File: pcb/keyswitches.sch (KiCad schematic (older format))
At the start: 59 parts, among them J5 Conn_01x05, J6 Conn_01x03, SW1 SW_PUSH, SW10 SW_PUSH, SW11 SW_PUSH, SW12 SW_PUSH, SW13 SW_PUSH, SW14 SW_PUSH, SW15 SW_PUSH, SW16 SW_PUSH, SW17 SW_PUSH, SW18 SW_PUSH, SW19 SW_PUSH, SW2 SW_PUSH, SW20 SW_PUSH, SW21 SW_PUSH, SW22 SW_PUSH, SW23 SW_PUSH, SW24 SW_PUSH, SW25 SW_PUSH, SW26 SW_PUSH, SW27 SW_PUSH, SW28 Rotary_Encoder, SW29 Rotary_Encoder, SW3 SW_PUSH, SW30 Rotary_Encoder, SW4 SW_PUSH, SW5 SW_PUSH, SW6 SW_PUSH, SW7 SW_PUSH, SW8 SW_PUSH, SW9 SW_PUSH

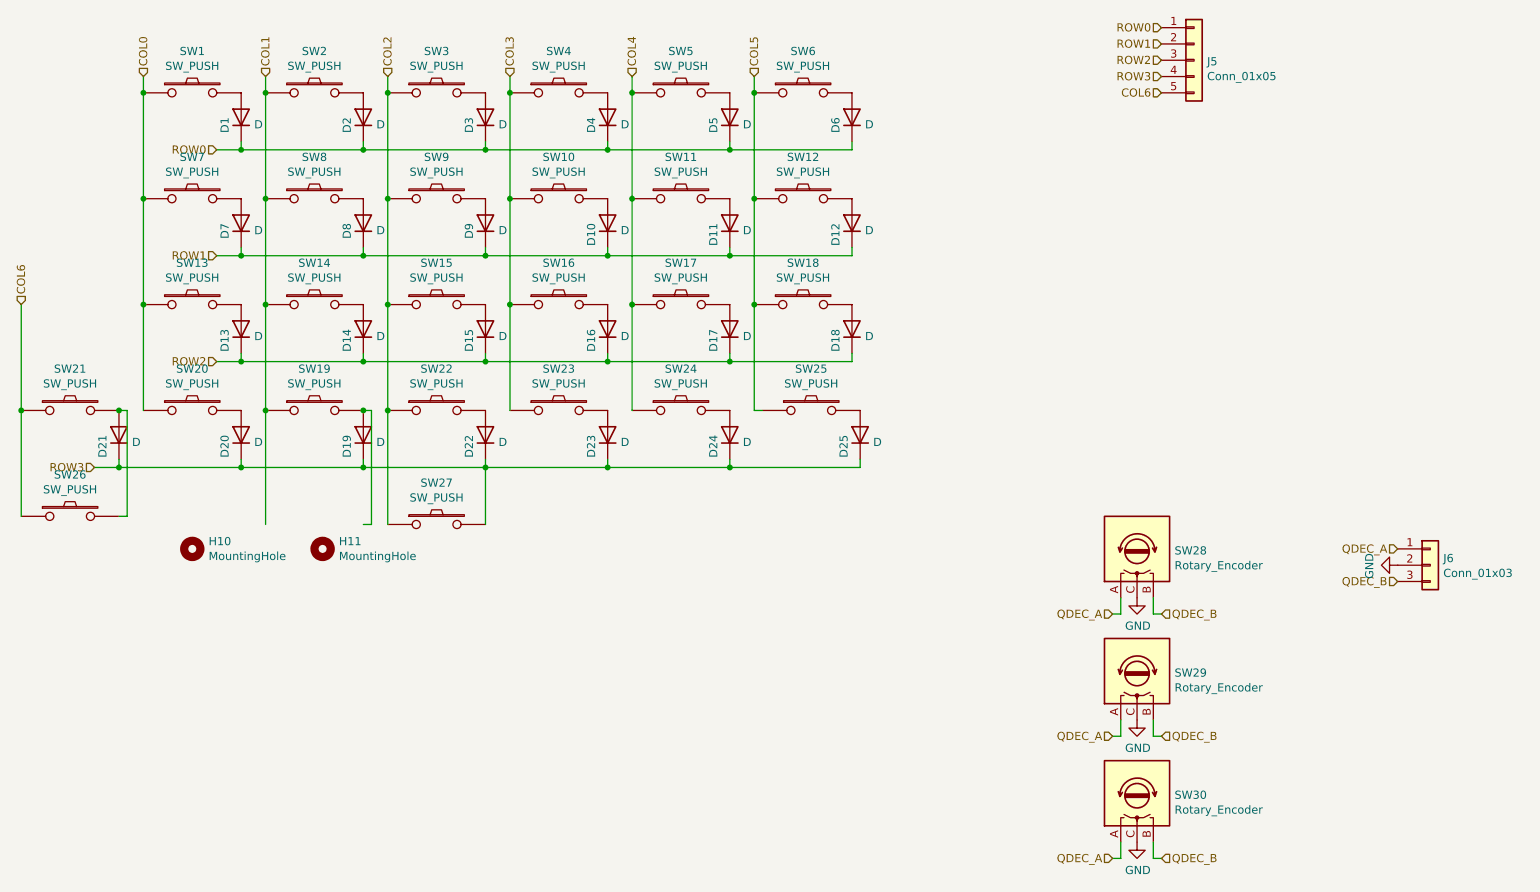
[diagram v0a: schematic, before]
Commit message: And another update
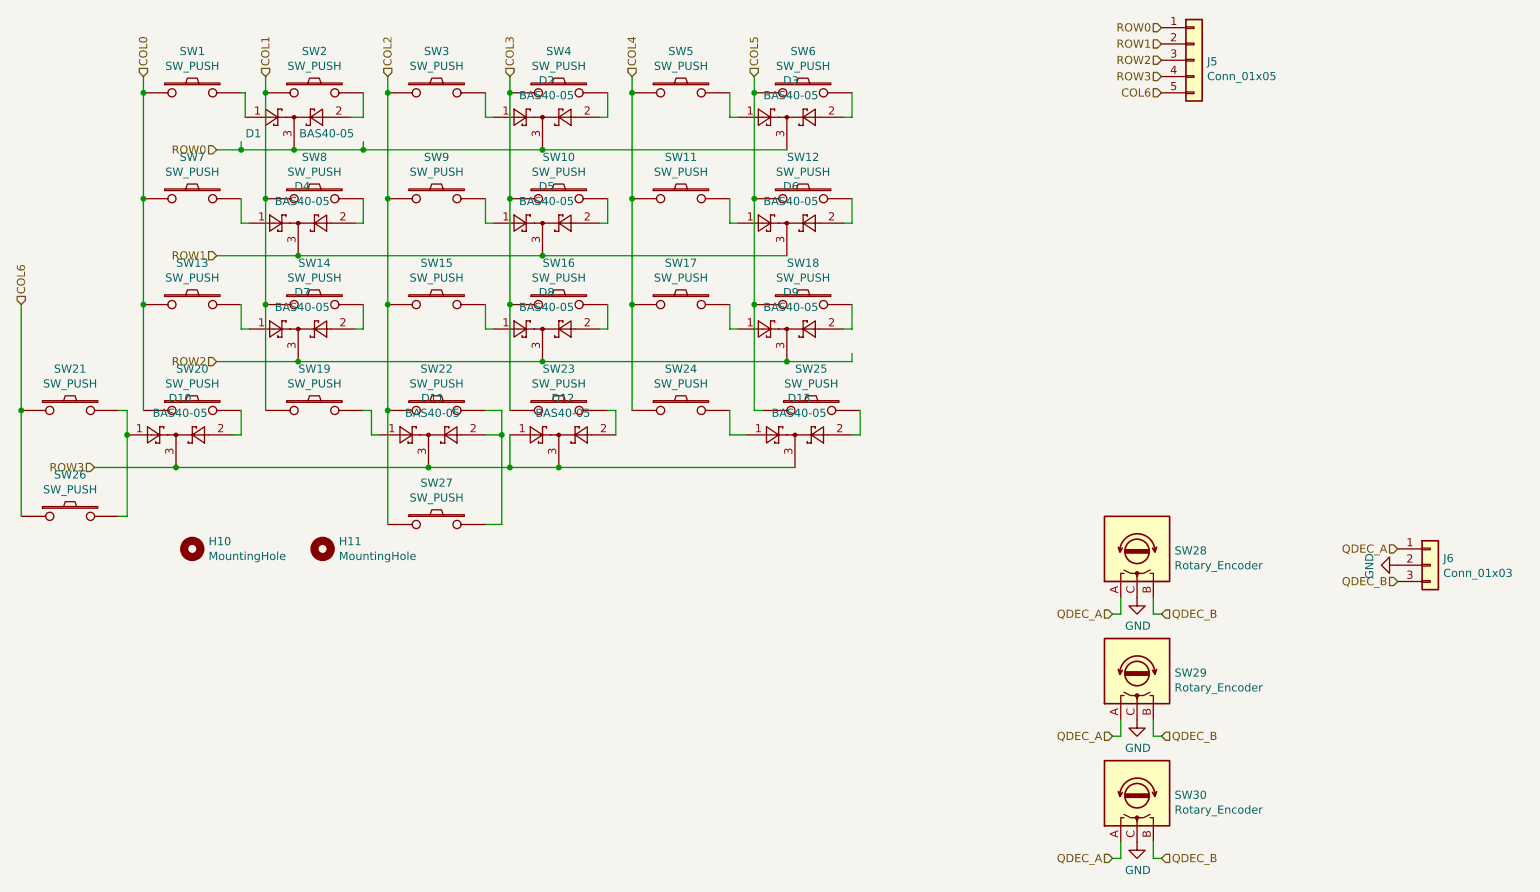
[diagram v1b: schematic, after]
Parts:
- removed D1, D10, D11, D12, D13, D14, D15, D16, D17, D18, D19, D2, D20, D21, D22, D23, D24, D25, D3, D4, D5, D6, D7, D8, D9: D, lib:D3_SMD_v2_mirror, symbol Device:D
- added D1, D10, D11, D12, D13, D2, D3, D4, D5, D6, D7, D8, D9: BAS40-05, lib:SOT-23_mirror, symbol lib:BAS40-05
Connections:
- net ROW0: now also D1.3, D2.3, D3.3
- net ROW1: now also D4.3, D5.3, D6.3
- net ROW2: now also D7.3, D8.3, D9.3
- net ROW3: now also D10.3, D11.3, D12.1, D12.3, D13.3; no longer SW27.2
- net at SW1.2: now also D1.1
- net at SW2.2: now also D1.2
- net at SW3.2: now also D2.1
- net at SW4.2: now also D2.2
- net at SW5.2: now also D3.1
- net at SW6.2: now also D3.2
- net at SW7.2: now also D4.1
- net at SW8.2: now also D4.2
- net at SW9.2: now also D5.1
- net at SW10.2: now also D5.2
- net at SW11.2: now also D6.1
- net at SW12.2: now also D6.2
- net at SW13.2: now also D7.1
- net at SW14.2: now also D7.2
- net at SW15.2: now also D8.1
- net at SW16.2: now also D8.2
- net at SW17.2: now also D9.1
- net at SW18.2: now also D9.2
- net at SW19.2: now also D11.1
- net at SW20.2: now also D10.2
- net at SW21.2, SW26.2: now also D10.1
- net at SW22.2: now also SW27.2, D11.2
- net at SW23.2: now also D12.2
- net at SW24.2: now also D13.1
- net at SW25.2: now also D13.2
